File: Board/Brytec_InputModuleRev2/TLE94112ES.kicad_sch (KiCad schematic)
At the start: 1 part, among them U9 TLE94112ES

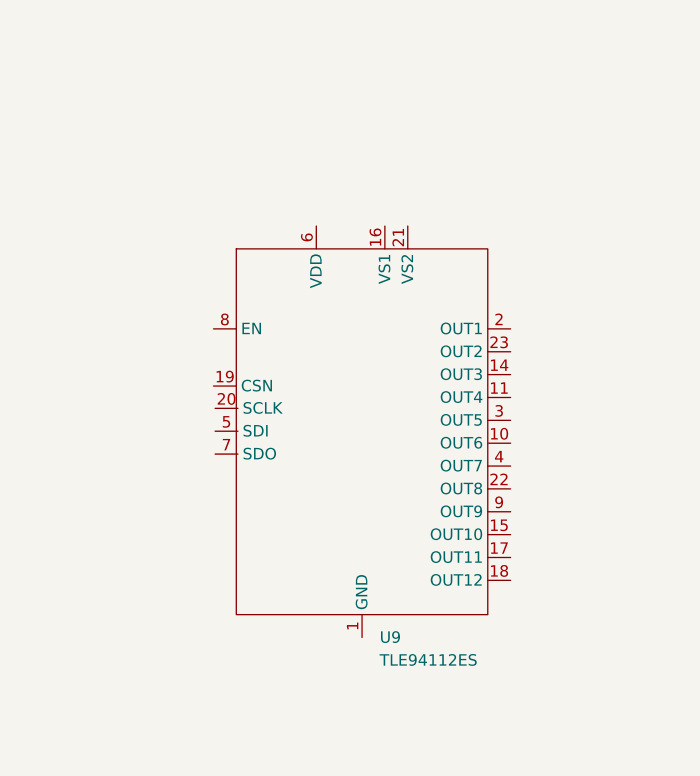
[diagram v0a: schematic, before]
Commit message: Updated board
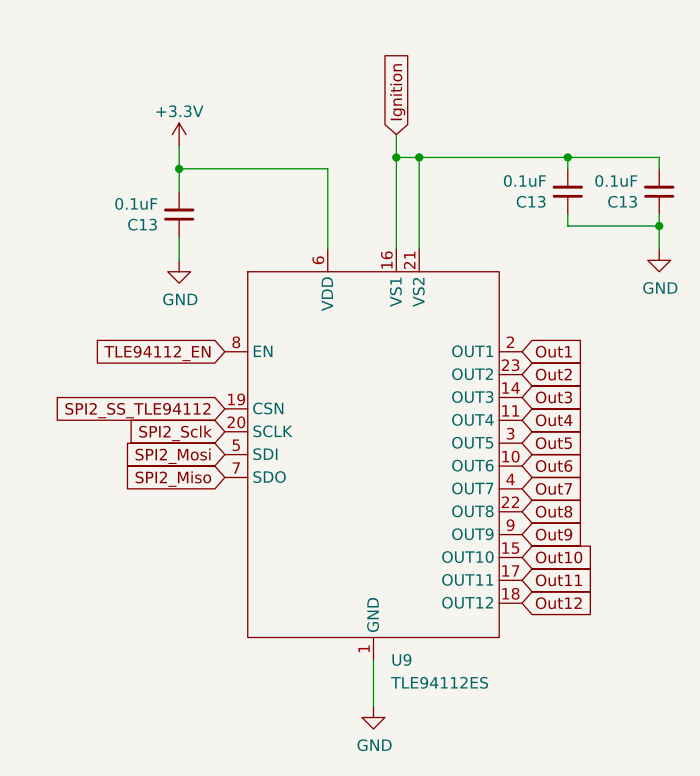
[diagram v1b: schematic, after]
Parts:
- added C13 (x3): 0.1uF, Capacitor_SMD:C_0603_1608Metric_Pad1.08x0.95mm_HandSolder, symbol Device:C_Small
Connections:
- net GND: now reaches U9.1 (GND), U9.12 (GND), U9.13 (GND), U9.24 (GND), U9.EDP (GND)
- net GND: now also C13.1, C13.1, C13.1
- net Out6: now reaches U9.10 (OUT6)
- net Out4: now reaches U9.11 (OUT4)
- net Out3: now reaches U9.14 (OUT3)
- net Out10: now reaches U9.15 (OUT10)
- net Ignition: now reaches U9.16 (VS1)
- net Ignition: now also U9.21 (VS2), C13.2, C13.2
- net Out11: now reaches U9.17 (OUT11)
- net Out12: now reaches U9.18 (OUT12)
- net SPI2_SS_TLE94112: now reaches U9.19 (CSN)
- net Out1: now reaches U9.2 (OUT1)
- net SPI2_Sclk: now reaches U9.20 (SCLK)
- net Out8: now reaches U9.22 (OUT8)
- net Out2: now reaches U9.23 (OUT2)
- net Out5: now reaches U9.3 (OUT5)
- net Out7: now reaches U9.4 (OUT7)
- net SPI2_Mosi: now reaches U9.5 (SDI)
- net +3.3V: now reaches U9.6 (VDD)
- net +3.3V: now also C13.2
- net SPI2_Miso: now reaches U9.7 (SDO)
- net TLE94112_EN: now reaches U9.8 (EN)
- net Out9: now reaches U9.9 (OUT9)
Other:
- moved on the sheet: U9
